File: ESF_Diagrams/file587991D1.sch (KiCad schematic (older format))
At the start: 8 parts

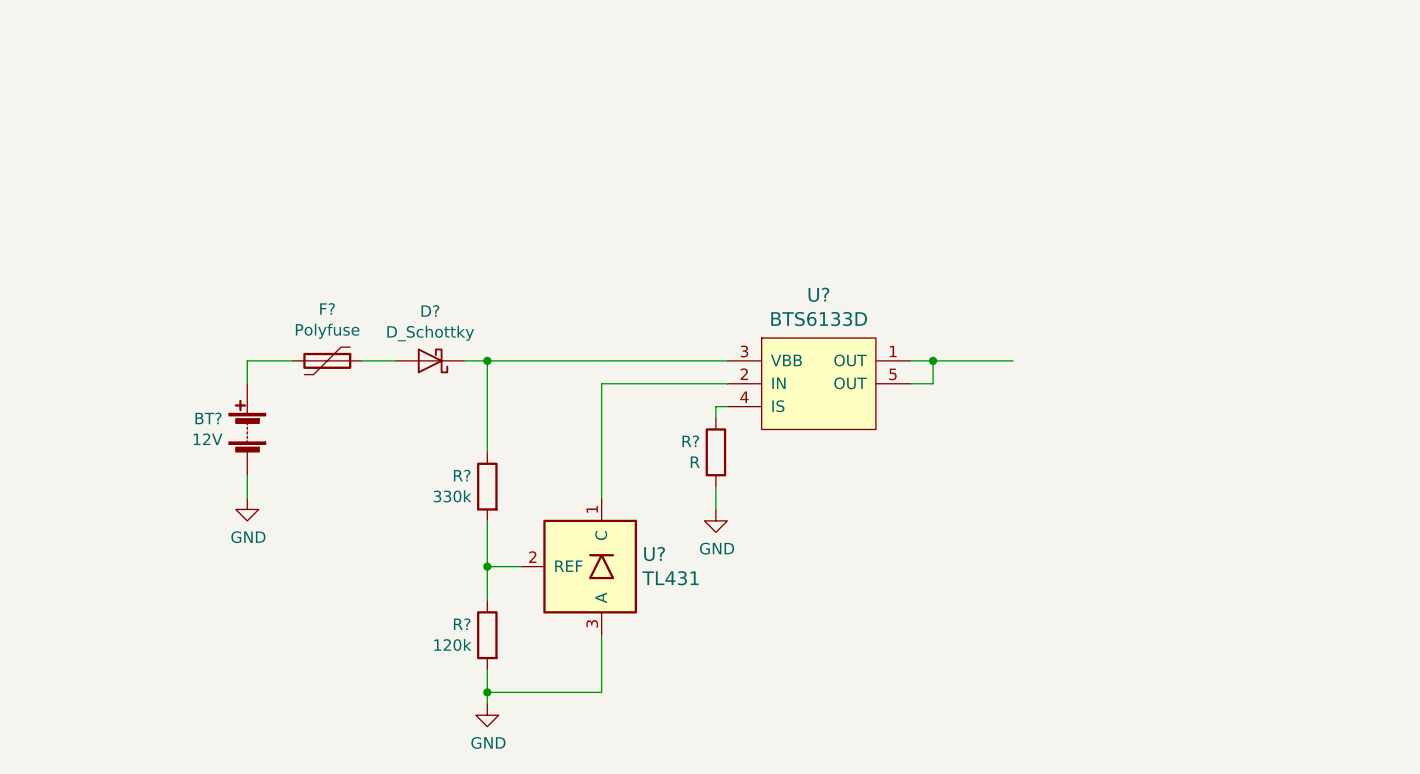
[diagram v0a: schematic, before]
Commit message: Updates all around
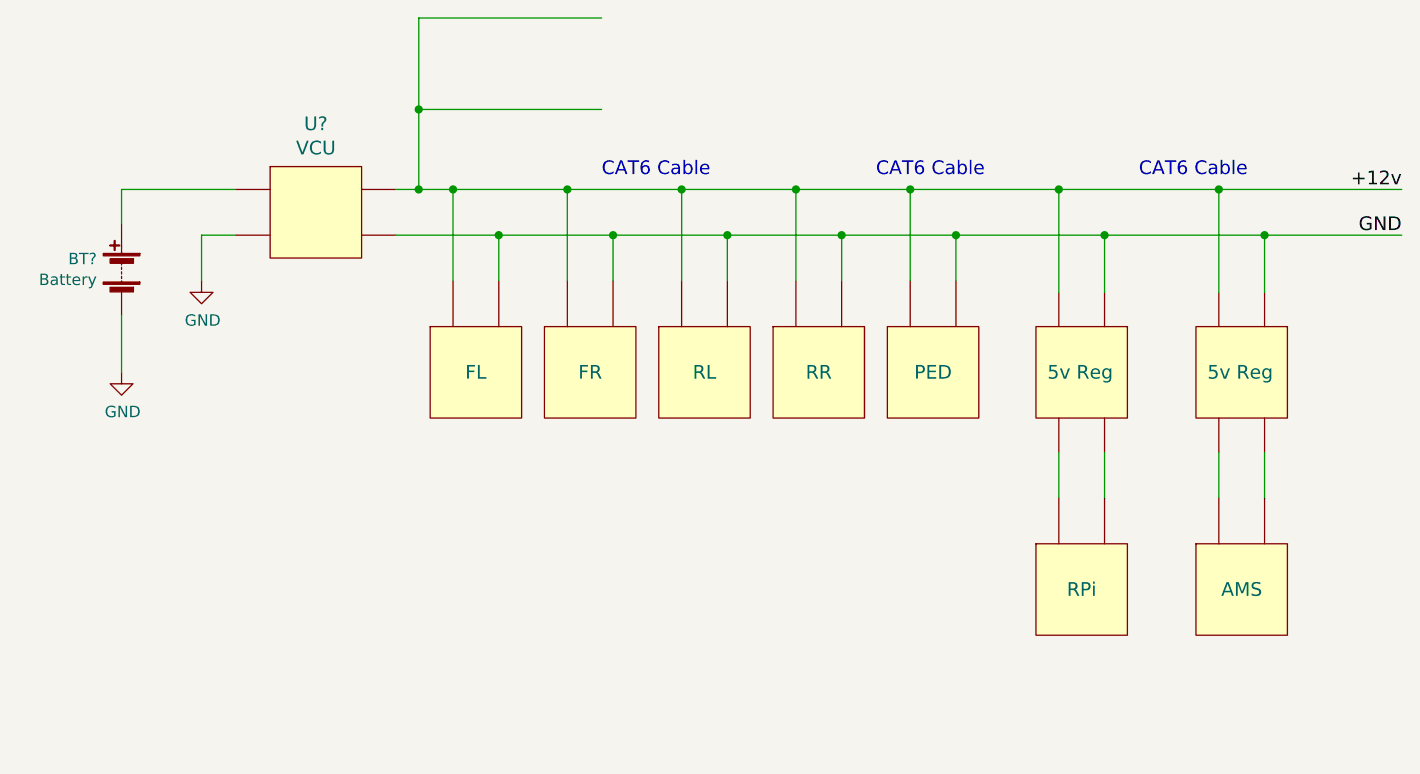
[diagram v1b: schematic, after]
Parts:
- removed BT?: 12V, symbol Battery
- removed D?: D_Schottky, symbol D_Schottky
- removed F?: Polyfuse, symbol Polyfuse
- removed R?: 330k, symbol R
- removed R?: 120k, symbol R
- removed R?: R, symbol R
- removed U?: TL431, symbol TL431
- removed U?: BTS6133D, symbol BTS6133D
- added BT?: Battery, symbol Battery
- added U?: VCU, symbol Generic_2x2
- added U?: FL, symbol Generic_CAN_Node
- added U?: FR, symbol Generic_CAN_Node
- added U?: RL, symbol Generic_CAN_Node
- added U?: RR, symbol Generic_CAN_Node
- added U?: PED, symbol Generic_CAN_Node
- added U?: RPi, symbol Generic_CAN_Node
- added U?: AMS, symbol Generic_CAN_Node
- added U? (x2): 5v Reg, symbol Generic_2x2
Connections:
- net labels added: +12v
- wire segments 23 -> 28
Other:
- note added: "CAT6 Cable"
